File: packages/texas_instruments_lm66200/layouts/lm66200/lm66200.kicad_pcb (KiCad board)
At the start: 2 copper layers, 4 parts

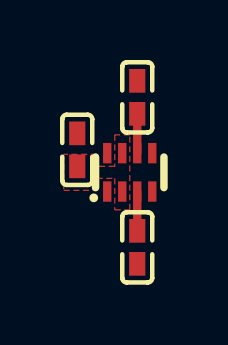
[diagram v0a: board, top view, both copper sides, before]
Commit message: WIP update lm66200
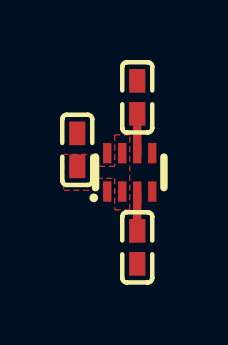
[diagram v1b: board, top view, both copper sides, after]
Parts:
- C1, C2, C3: footprint atopile:C0402-b3ef17 -> Samsung_Electro_Mechanics_CL05B104KO5NNNC:C0402
- U1: footprint atopile:SOT-583-8_L2.1-W1.2-P0.50-LS1.6-BL-f9e8a4 -> Texas_Instruments_LM66200DRLR:SOT-583-8_L2.1-W1.2-P0.50-LS1.6-BL
